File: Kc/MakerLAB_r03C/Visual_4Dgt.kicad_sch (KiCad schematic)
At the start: 15 parts, among them J11 Conn_02x10_Counter_Clockwise, J12 Conn_02x05_Counter_Clockwise, J9 Conn_02x05_Counter_Clockwise, Q1 2N3904, Q2 2N3904, Q3 2N3904, Q4 2N3904, U3 DM9368, U4 CC56-12EWA

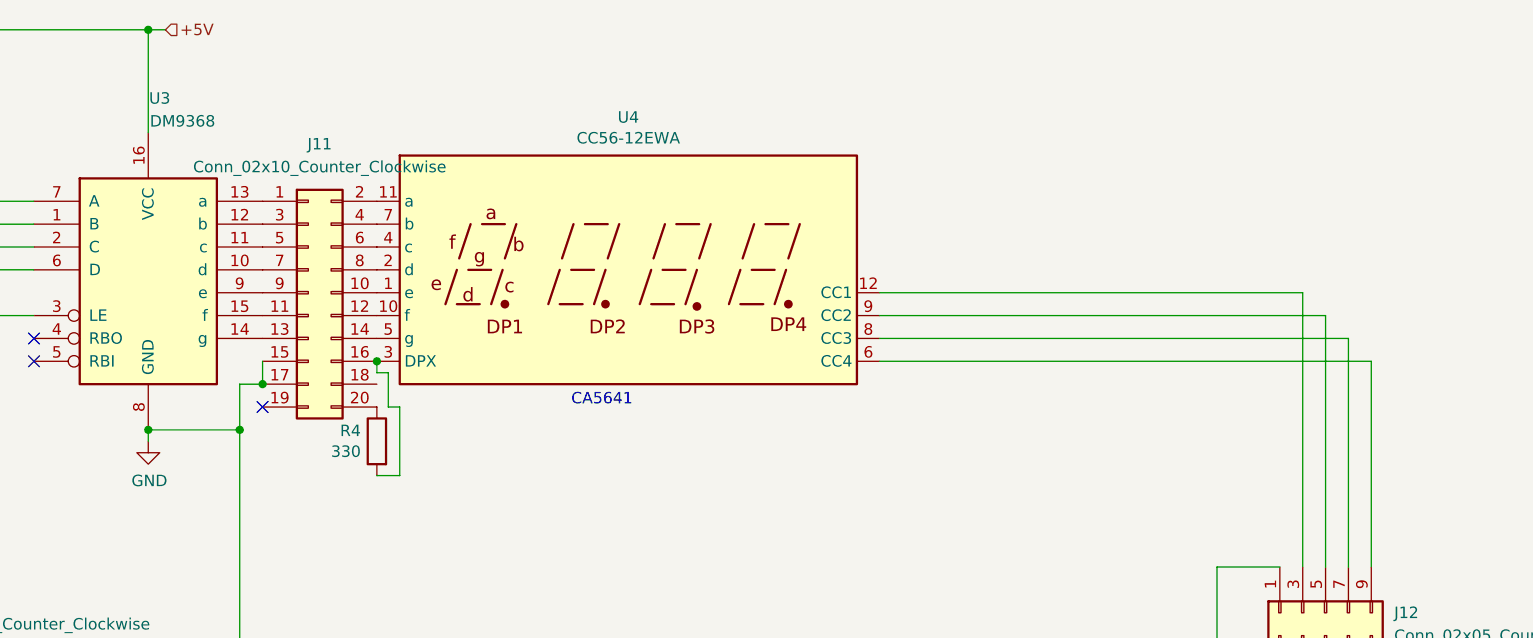
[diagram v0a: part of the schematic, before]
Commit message: 20230404 14:30
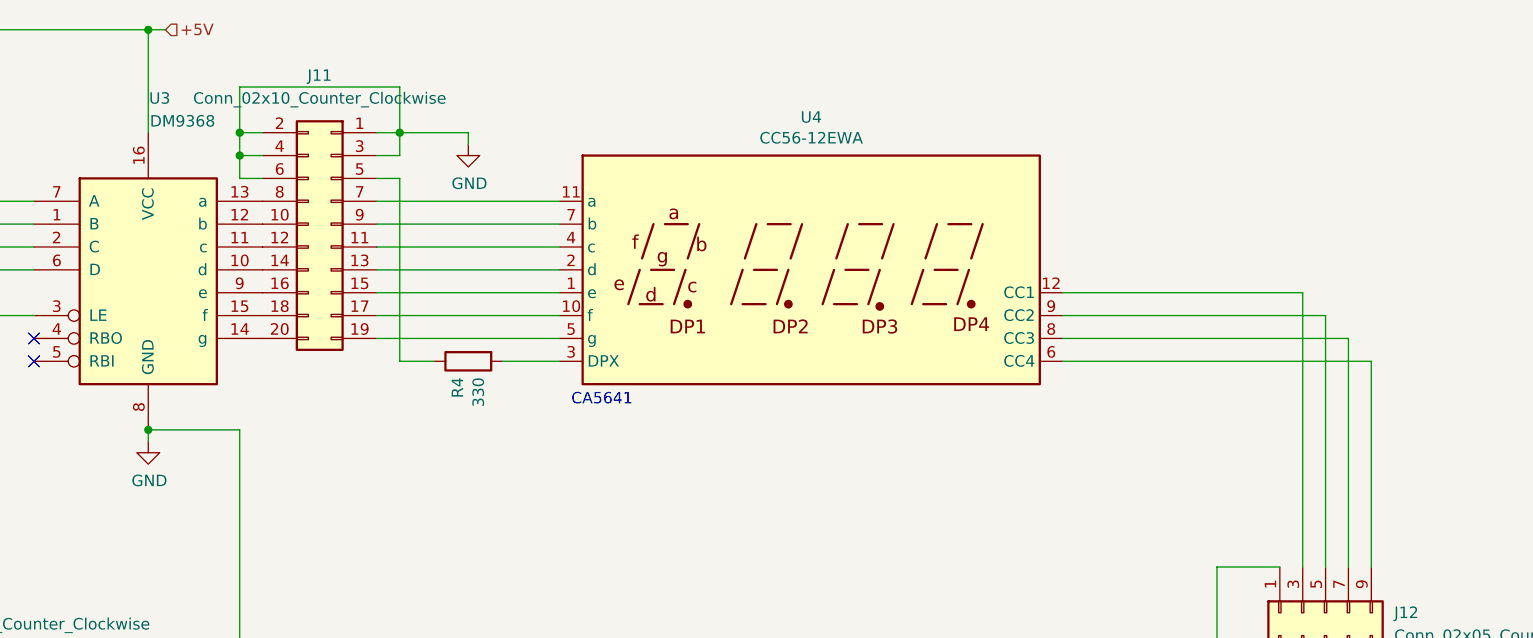
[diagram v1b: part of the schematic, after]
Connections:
- net GND: now also J11.1 (Pin_1), J11.2 (Pin_2), J11.3 (Pin_3), J11.4 (Pin_4), J11.6 (Pin_6); no longer J11.15 (Pin_15), J11.17 (Pin_17)
- net at U4.1 (e): now also J11.15 (Pin_15); no longer J11.10 (Pin_10)
- net at U4.10 (f): now also J11.17 (Pin_17); no longer J11.12 (Pin_12)
- net at U4.11 (a): now also J11.7 (Pin_7); no longer J11.2 (Pin_2)
- net at U4.2 (d): now also J11.13 (Pin_13); no longer J11.8 (Pin_8)
- net at R4.2, U4.3 (DPX): no longer J11.16 (Pin_16)
- net at U4.4 (c): now also J11.11 (Pin_11); no longer J11.6 (Pin_6)
- net at U4.5 (g): now also J11.19 (Pin_19); no longer J11.14 (Pin_14)
- net at U4.7 (b): now also J11.9 (Pin_9); no longer J11.4 (Pin_4)
- net at U3.13 (a): now also J11.8 (Pin_8); no longer J11.1 (Pin_1)
- net at U3.15 (f): now also J11.18 (Pin_18); no longer J11.11 (Pin_11)
- net at U3.14 (g): now also J11.20 (Pin_20); no longer J11.13 (Pin_13)
- net at R4.1: now also J11.5 (Pin_5); no longer J11.20 (Pin_20)
- net at U3.12 (b): now also J11.10 (Pin_10); no longer J11.3 (Pin_3)
- net at U3.11 (c): now also J11.12 (Pin_12); no longer J11.5 (Pin_5)
- net at U3.10 (d): now also J11.14 (Pin_14); no longer J11.7 (Pin_7)
- net at U3.9 (e): now also J11.16 (Pin_16); no longer J11.9 (Pin_9)
- no-connect marks 3 -> 2
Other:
- moved on the sheet: J11, R4, U4
